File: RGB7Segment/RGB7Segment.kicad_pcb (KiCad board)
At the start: 2 copper layers, 1.4 x 2.4 mm, 21 parts, among them J1 Conn_01x02_Socket, J2 Conn_01x02_Socket

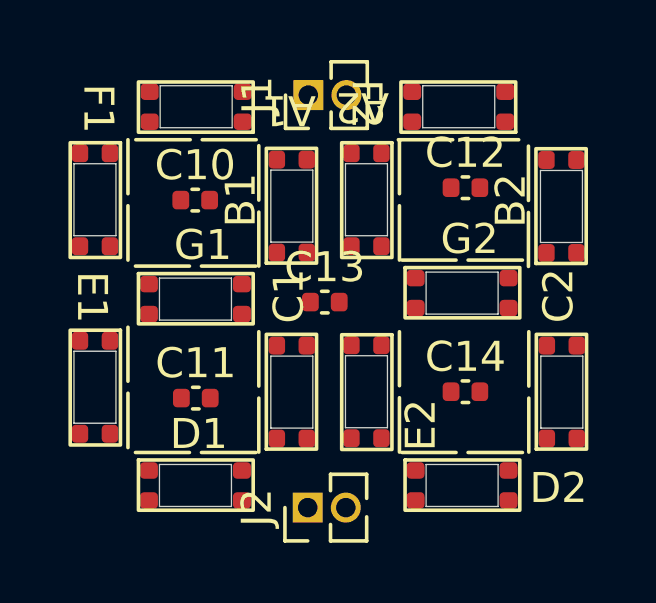
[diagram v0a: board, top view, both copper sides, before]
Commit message: New Layout possibility
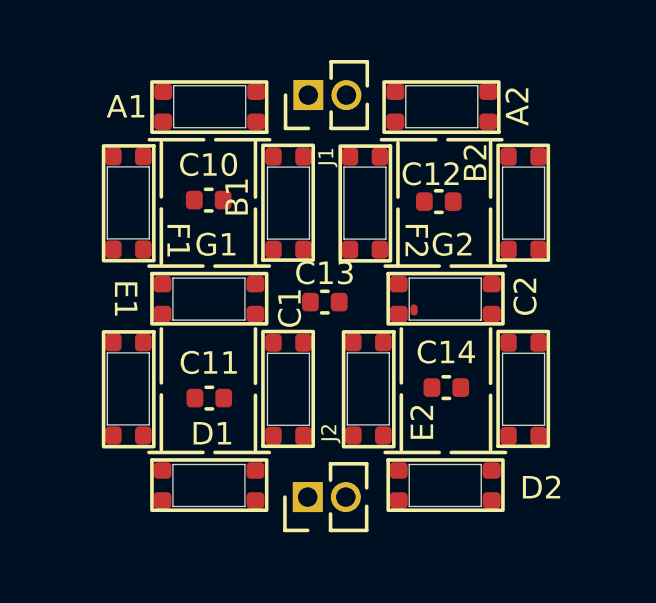
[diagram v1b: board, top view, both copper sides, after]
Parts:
- moved C2 1.28 mm to (208.9, 87.7)
- moved B2 1.27 mm to (208.9, 81.5)
- moved F1 1.12 mm to (194.8, 78.7)
- moved E1 1.11 mm to (194.8, 84.9)
- moved C12 1.00 mm to (205.6, 80.0)
- moved C14 0.65 mm to (205.8, 86.2)
- moved G2 0.60 mm to (204.5, 83.8)
- moved A2 0.56 mm to (207.1, 76.4)
- moved D2 0.56 mm to (204.5, 90.0)
- moved C10 0.45 mm to (197.9, 80.0)
- moved D1 0.45 mm to (196.6, 90.0)
- moved G1 0.45 mm to (196.6, 83.8)
- moved A1 0.45 mm to (199.3, 76.4)
- moved C11 0.45 mm to (197.9, 86.6)
- moved J2 0.35 mm to (201.2, 89.9)
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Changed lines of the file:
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@@
 	(footprint "Library:12-23C"
 		(layer "F.Cu")
-		(at 210.137501 81.5625 90)
+		(at 208.875 81.45 90)
 		(property "Reference" "B2"
-			(at 1.55 -2.137501 90)
+			(at 2.7 -2.0375 90)
 			(unlocked yes)
 			(layer "F.SilkS")
 			(effects
 				(font
-					(size 1 1)
+					(size 0.75 0.75)
 					(thickness 0.15)
 				)
@@
 	(footprint "Library:12-23C"
 		(layer "F.Cu")
-		(at 196.1375 83.75)
+		(at 196.5875 83.75)
 		(property "Reference" "G1"
 			(at 1.6 -2.25 0)
@@
 			(effects
 				(font
-					(size 1 1)
+					(size 0.75 0.75)
 					(thickness 0.15)
 				)
@@
 	(footprint "Library:12-23C"
 		(layer "F.Cu")
-		(at 196.1375 89.9625)
+		(at 196.5875 89.9625)
 		(property "Reference" "D1"
 			(at 1.4625 -2.1625 0)
@@
 			(effects
 				(font
-					(size 1 1)
+					(size 0.75 0.75)
 					(thickness 0.15)
 				)
@@
 	(footprint "Library:12-23C"
 		(layer "F.Cu")
-		(at 207.6125 76.4375 180)
+		(at 207.05 76.4375 180)
 		(property "Reference" "A2"
-			(at 4.575 -0.462499 180)
+			(at -1.1875 -0.4125 90)
 			(unlocked yes)
 			(layer "F.SilkS")
 			(effects
 				(font
-					(size 1 1)
+					(size 0.75 0.75)
 					(thickness 0.15)
 				)
@@
 		(tags "Through hole pin header THT 1x02 1.27mm single row")
 		(property "Reference" "J1"
-			(at 0 -1.695 90)
+			(at -2.05 0.6 -90)
 			(layer "F.SilkS")
 			(effects
 				(font
-					(size 1 1)
-					(thickness 0.15)
+					(size 0.5 0.5)
+					(thickness 0.125)
 				)
 			)
@@
 	(footprint "Capacitor_SMD:C_0402_1005Metric"
 		(layer "F.Cu")
-		(at 206.4875 79.5875)
+		(at 205.6 80.05)
 		(descr "Capacitor SMD 0402 (1005 Metric), square (rectangular) end terminal, IPC_7351 nominal, (Body size source: IPC-SM-782 page 76, https://www.pcb-3d.com/wordpress/wp-content/uploads/ipc-sm-782a_amendment_1_and_2.pdf), generated with kicad-footprint-generator")
 		(tags "capacitor")
 		(property "Reference" "C12"
-			(at 0 -1.16 0)
+			(at -0.25 -0.9 0)
 			(layer "F.SilkS")
 			(effects
 				(font
-					(size 1 1)
+					(size 0.75 0.75)
 					(thickness 0.15)
 				)
@@
 	(footprint "Library:12-23C"
 		(layer "F.Cu")
-		(at 205.025 83.55)
+		(at 204.4625 83.75)
 		(property "Reference" "G2"
 			(at 1.6 -2.25 0)
@@
 			(effects
 				(font
-					(size 1 1)
+					(size 0.75 0.75)
 					(thickness 0.15)
 				)
@@
 	(footprint "Connector_PinHeader_1.27mm:PinHeader_1x02_P1.27mm_Vertical"
 		(layer "F.Cu")
-		(at 201.229999 90.25 90)
+		(at 201.23 89.9 90)
 		(descr "Through hole straight pin header, 1x02, 1.27mm pitch, single row")
 		(tags "Through hole pin header THT 1x02 1.27mm single row")
 		(property "Reference" "J2"
-			(at 0 -1.695 90)
+			(at 2.15 0.72 270)
 			(layer "F.SilkS")
 			(effects
 				(font
-					(size 1 1)
-					(thickness 0.15)
+					(size 0.5 0.5)
+					(thickness 0.125)
 				)
 			)
@@
 		(tags "capacitor")
 		(property "Reference" "C13"
-			(at 0 -1.16 0)
+			(at 0 -0.95 0)
 			(layer "F.SilkS")
 			(effects
 				(font
-					(size 1 1)
+					(size 0.75 0.75)
 					(thickness 0.15)
 				)
@@
 	(footprint "Library:12-23C"
 		(layer "F.Cu")
-		(at 202.7375 78.6375 -90)
+		(at 202.6875 78.75 -90)
 		(property "Reference" "F2"
-			(at -1.8375 -0.45 -90)
+			(at 2.6 -2.15 270)
 			(unlocked yes)
 			(layer "F.SilkS")
 			(effects
 				(font
-					(size 1 1)
+					(size 0.75 0.75)
 					(thickness 0.15)
 				)
@@
 	(footprint "Library:12-23C"
 		(layer "F.Cu")
-		(at 193.6875 84.8875 -90)
+		(at 194.8 84.94375 -90)
 		(property "Reference" "E1"
-			(at -1.65 -0.35 -90)
+			(at -1.65 -0.35 270)
 			(unlocked yes)
 			(layer "F.SilkS")
 			(effects
 				(font
-					(size 1 1)
+					(size 0.75 0.75)
 					(thickness 0.15)
 				)
@@
 	(footprint "Capacitor_SMD:C_0402_1005Metric"
 		(layer "F.Cu")
-		(at 206.4875 86.3875)
+		(at 205.85 86.25)
 		(descr "Capacitor SMD 0402 (1005 Metric), square (rectangular) end terminal, IPC_7351 nominal, (Body size source: IPC-SM-782 page 76, https://www.pcb-3d.com/wordpress/wp-content/uploads/ipc-sm-782a_amendment_1_and_2.pdf), generated with kicad-footprint-generator")
 		(tags "capacitor")
@@
 			(effects
 				(font
-					(size 1 1)
+					(size 0.75 0.75)
 					(thickness 0.15)
 				)
@@
 	(footprint "Capacitor_SMD:C_0402_1005Metric"
 		(layer "F.Cu")
-		(at 197.48 80)
+		(at 197.93 80)
 		(descr "Capacitor SMD 0402 (1005 Metric), square (rectangular) end terminal, IPC_7351 nominal, (Body size source: IPC-SM-782 page 76, https://www.pcb-3d.com/wordpress/wp-content/uploads/ipc-sm-782a_amendment_1_and_2.pdf), generated with kicad-footprint-generator")
 		(tags "capacitor")
@@
 			(effects
 				(font
-					(size 1 1)
+					(size 0.75 0.75)
 					(thickness 0.15)
 				)
@@
 	(footprint "Library:12-23C"
 		(layer "F.Cu")
-		(at 198.8625 76.4375 180)
+		(at 199.3125 76.4375 180)
 		(property "Reference" "A1"
-			(at -1.7375 -0.562501 180)
+			(at 4.1125 -0.4625 0)
 			(unlocked yes)
 			(layer "F.SilkS")
 			(effects
 				(font
-					(size 1 1)
+					(size 0.75 0.75)
 					(thickness 0.15)
 				)
@@
 	(footprint "Library:12-23C"
 		(layer "F.Cu")
-		(at 201.149999 81.55 90)
+		(at 201.0375 81.45 90)
 		(property "Reference" "B1"
 			(at 1.55 -2.149999 90)
@@
 			(effects
 				(font
-					(size 1 1)
+					(size 0.75 0.75)
 					(thickness 0.15)
 				)
@@
 	(footprint "Library:12-23C"
 		(layer "F.Cu")
-		(at 205.025 89.9625)
+		(at 204.4625 89.9625)
 		(property "Reference" "D2"
 			(at 4.5625 -0.3625 0)
@@
 			(effects
 				(font
-					(size 1 1)
+					(size 0.75 0.75)
 					(thickness 0.15)
 				)
@@
 	(footprint "Library:12-23C"
 		(layer "F.Cu")
-		(at 210.15 87.75 90)
+		(at 208.875 87.65625 90)
 		(property "Reference" "C2"
-			(at 4.5625 -0.5625 90)
+			(at 4.45625 -0.375 90)
 			(unlocked yes)
 			(layer "F.SilkS")
 			(effects
 				(font
-					(size 1 1)
+					(size 0.75 0.75)
 					(thickness 0.15)
 				)
@@
 	(footprint "Library:12-23C"
 		(layer "F.Cu")
-		(at 193.6875 78.6375 -90)
+		(at 194.8 78.74375 -90)
 		(property "Reference" "F1"
-			(at -1.6875 -0.5625 -90)
+			(at 2.60625 -2.1 270)
 			(unlocked yes)
 			(layer "F.SilkS")
 			(effects
 				(font
-					(size 1 1)
+					(size 0.75 0.75)
 					(thickness 0.15)
 				)
@@
 	(footprint "Library:12-23C"
 		(layer "F.Cu")
-		(at 202.7375 85.0375 -90)
+		(at 202.8 84.94375 -90)
 		(property "Reference" "E2"
 			(at 2.4625 -2.2625 90)
@@
 			(effects
 				(font
-					(size 1 1)
+					(size 0.75 0.75)
 					(thickness 0.15)
 				)
@@
 	(footprint "Library:12-23C"
 		(layer "F.Cu")
-		(at 201.149999 87.75 90)
+		(at 201.0375 87.65625 90)
 		(property "Reference" "C1"
-			(at 4.55 -0.549999 90)
+			(at 4.05625 -0.3875 90)
 			(unlocked yes)
 			(layer "F.SilkS")
 			(effects
 				(font
-					(size 1 1)
+					(size 0.75 0.75)
 					(thickness 0.15)
 				)
@@
 	(footprint "Capacitor_SMD:C_0402_1005Metric"
 		(layer "F.Cu")
-		(at 197.5 86.6)
+		(at 197.95 86.6)
 		(descr "Capacitor SMD 0402 (1005 Metric), square (rectangular) end terminal, IPC_7351 nominal, (Body size source: IPC-SM-782 page 76, https://www.pcb-3d.com/wordpress/wp-content/uploads/ipc-sm-782a_amendment_1_and_2.pdf), generated with kicad-footprint-generator")
 		(tags "capacitor")
@@
 			(effects
 				(font
-					(size 1 1)
+					(size 0.75 0.75)
 					(thickness 0.15)
 				)
@@
 	)
 	(segment
-		(start 210.187501 81.8125)
-		(end 210.187501 81.887501)
-		(width 0.25)
-		(layer "F.Cu")
-		(net 1)
-	)
-	(segment
-		(start 210.187501 81.8125)
-		(end 210.187501 81.937501)
-		(width 0.25)
-		(layer "F.Cu")
-		(net 1)
-	)
-	(segment
